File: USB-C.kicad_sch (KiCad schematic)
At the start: 36 parts, among them IC2 TPS2557QDRBTQ1, IC5 TPS2557QDRBTQ1, IC7 TPS2557QDRBTQ1, J10 USB_C_Receptacle, J5 USB_C_Receptacle_USB2.0_16P, J7 USB_C_Receptacle_USB2.0_16P

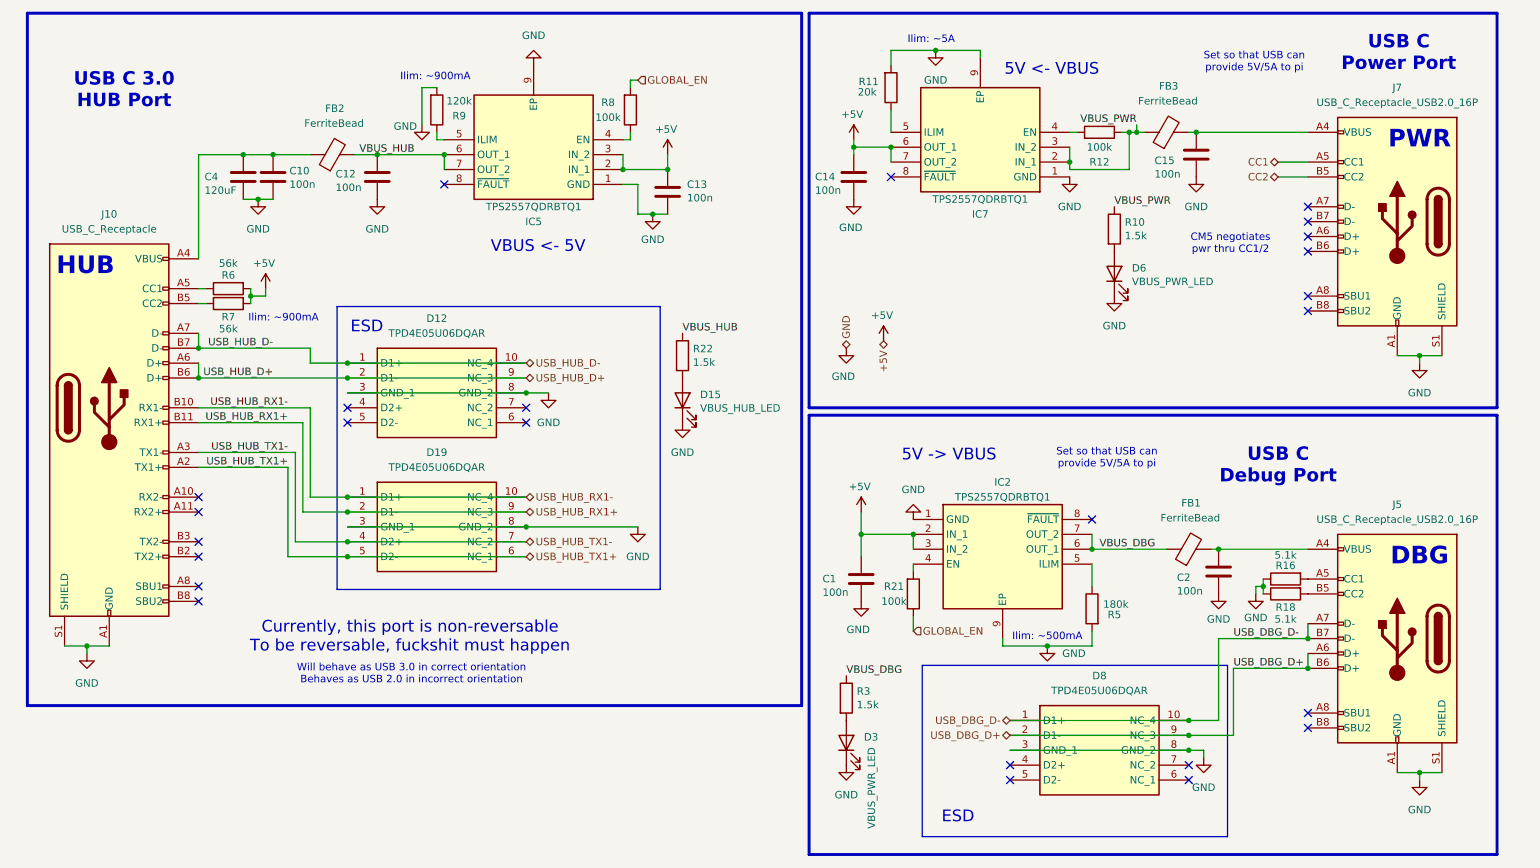
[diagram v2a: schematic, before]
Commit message: I hate my life
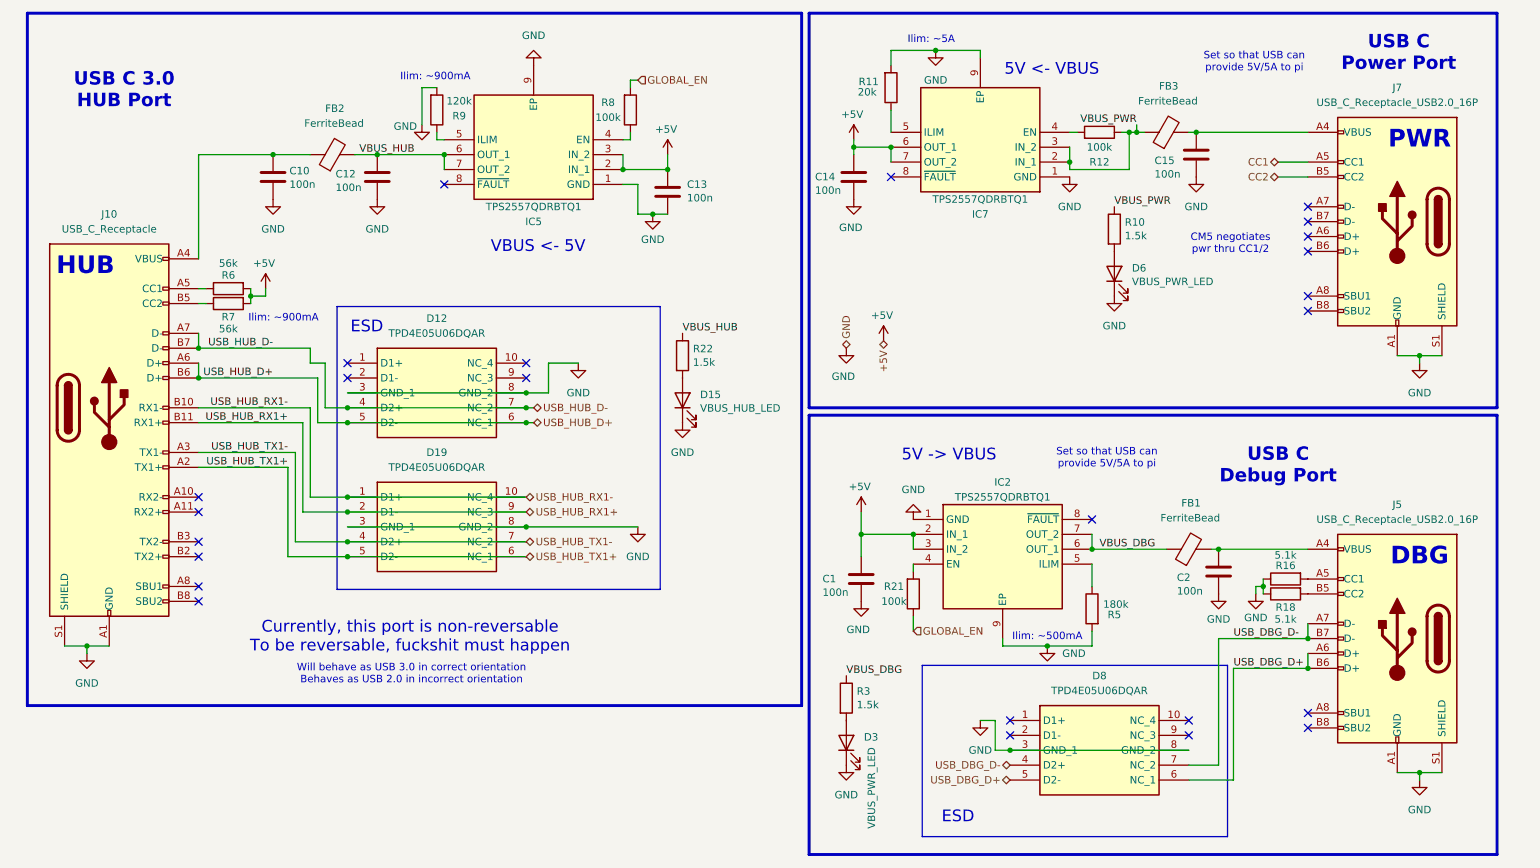
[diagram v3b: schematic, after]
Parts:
- removed C4: 120uF, Capacitor_SMD:C_0603_1608Metric, symbol Device:C
- C1, C10, C12, C13, C14, C15, C2: footprint Capacitor_SMD:C_0603_1608Metric -> Capacitor_SMD:C_0603_1608Metric_Pad1.08x0.95mm_HandSolder
- D15, D3, D6: footprint LED_SMD:LED_0603_1608Metric -> LED_SMD:LED_0603_1608Metric_Pad1.05x0.95mm_HandSolder
- R10, R11, R12, R16, R18, R21, R22, R3, R5, R6, R7, R8, R9: footprint Resistor_SMD:R_0603_1608Metric -> Resistor_SMD:R_0603_1608Metric_Pad0.98x0.95mm_HandSolder
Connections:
- net USB_DBG_D+: now also D8.5 (D2-), D8.6 (NC_1); no longer D8.2 (D1-), D8.9 (NC_3)
- net USB_DBG_D-: now also D8.4 (D2+), D8.7 (NC_2); no longer D8.1 (D1+), D8.10 (NC_4)
- net USB_HUB_D+: now also D12.5 (D2-), D12.6 (NC_1); no longer D12.2 (D1-), D12.9 (NC_3)
- net USB_HUB_D-: now also D12.4 (D2+), D12.7 (NC_2); no longer D12.1 (D1+), D12.10 (NC_4)
